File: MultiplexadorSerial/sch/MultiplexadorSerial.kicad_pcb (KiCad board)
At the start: 2 copper layers, 69.2 x 54 mm, 65 parts, among them J1 SL4, J2 SL3, J3 SL1, J4 SL2, Q1 Q_NPN_CBE, Q2 Q_NPN_CBE, Q3 Q_NPN_CBE, Q4 Q_NPN_CBE, U1 SP3481CP, U2 SP3481CP, U3 SP3481CP, U4 SP3481CP, U5 4052

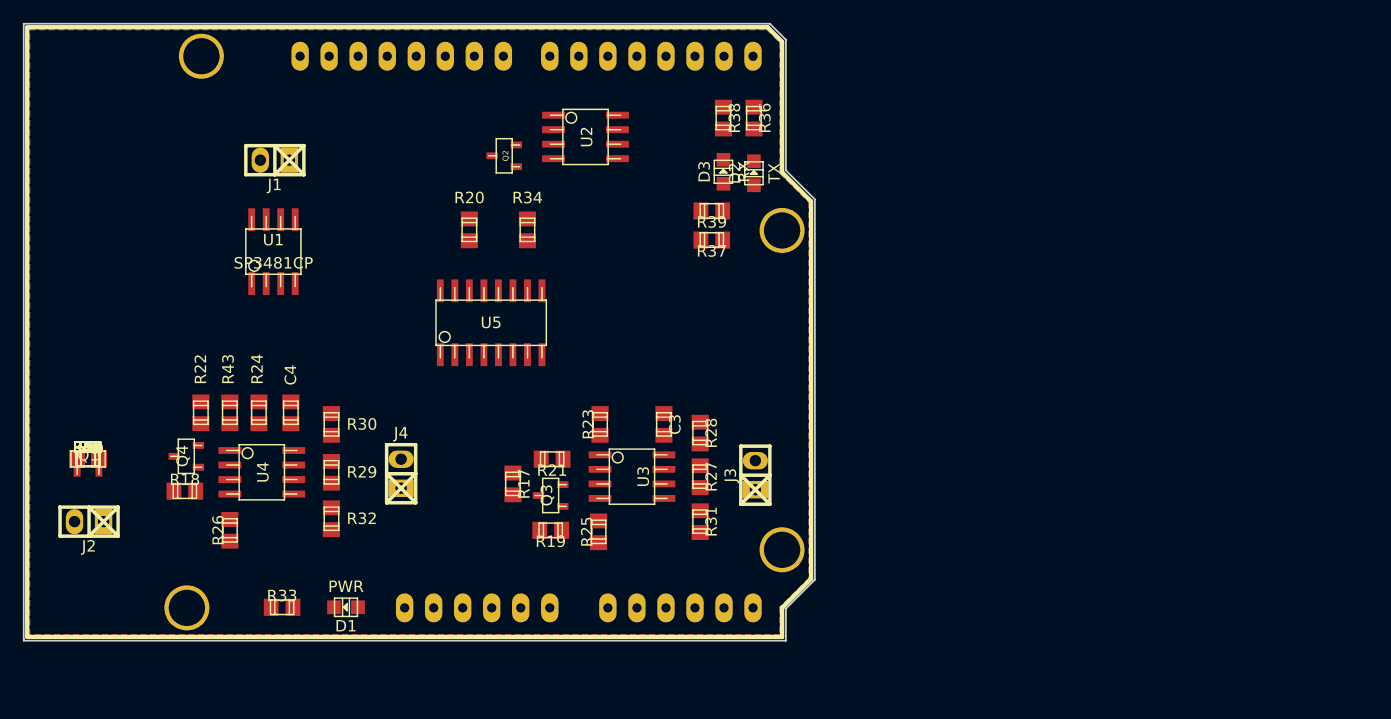
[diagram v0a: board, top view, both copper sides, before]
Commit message: novo desenho
Signed-off-by: cuki2 <mauricio@krebs.com.br>
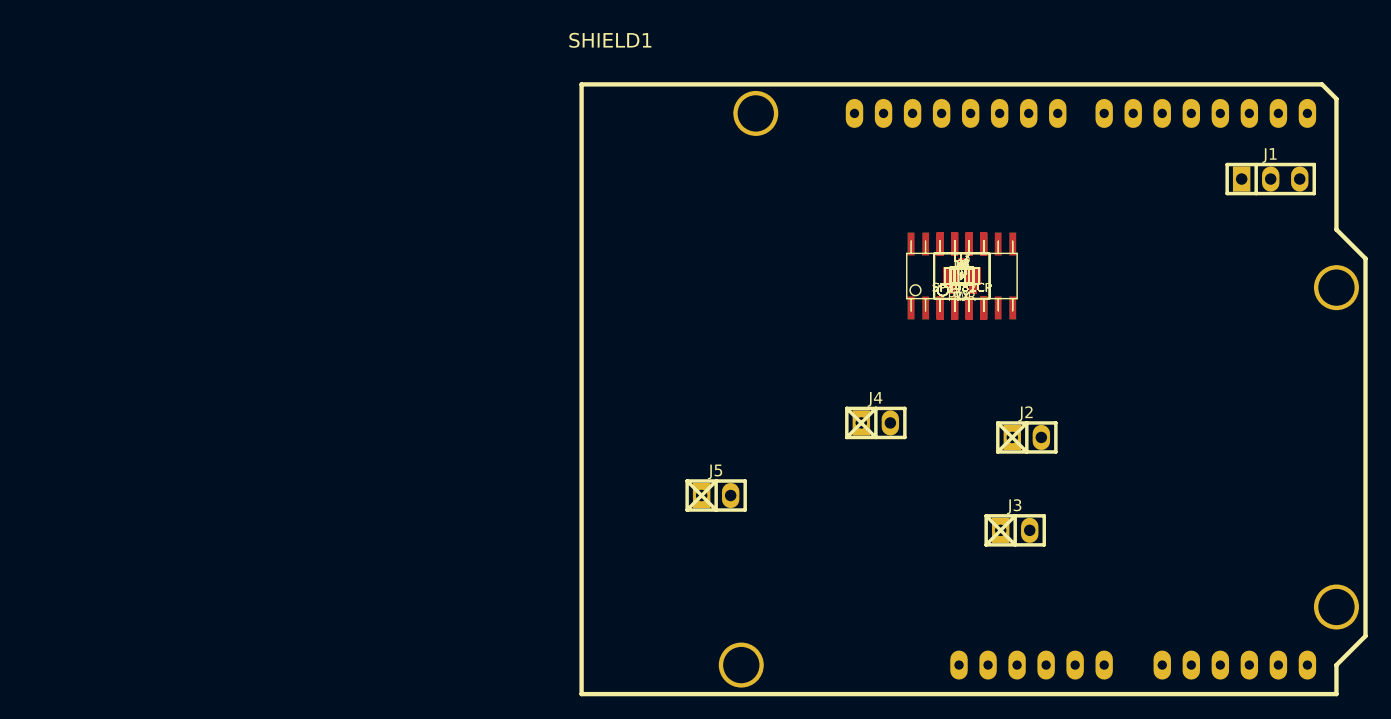
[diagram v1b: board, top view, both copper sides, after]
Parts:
- added J5: SL4, w_pin_strip:pin_socket_2, F.Cu at (160.3, 87.6)
- added R44, R45: 560R, w_smd_resistors:r_0805, F.Cu at (181.8, 68.4)
- D1: value PWR -> TX
- D2: value TX -> PWR
- J1: value SL4 -> SL; footprint w_pin_strip:pin_socket_2 -> w_pin_strip:pin_socket_3
- J2: value SL3 -> SL1
- J3: value SL1 -> SL2
- J4: value SL2 -> SL3
- R1, R2: value 10k -> 1k2
- R10, R18, R26: value 10k -> 560R
- R11, R27: value 120R -> 560R
- R12, R16: value 560R -> 330R
- R13: value 120R -> 330R
- R14, R15, R19, R20, R24, R28, R3, R30, R39, R4, R8: value 560R -> 10k
- R17: value 10k -> 330R
- R22, R40, R41, R6: value 10k -> 360R
- R23, R31, R32, R7: value 560R -> 360R
- R25, R43, R9: value 10k -> 120R
- R29: value 120R -> 10k
- R33, R37: value 1k2 -> 10k
- R34: value 330R -> 120R
- R35, R36: value 330R -> 560R
- R38: value 330R -> 10k
- U2: value SP3481CP -> 4052; footprint w_smd_dil:so-8 -> w_smd_dil:so-16
- U5: value 4052 -> SP3481CP; footprint w_smd_dil:so-16 -> w_smd_dil:so-8
- moved J1 87.1 mm to (208.8, 59.9), turned to 0 degrees
- moved J2 82.4 mm to (187.5, 82.5), turned to 0 degrees
- moved C1 78.1 mm to (181.8, 68.4)
- moved C2 78.1 mm to (181.8, 68.4)
- moved C5 78.1 mm to (181.8, 68.4)
- moved Q1 78.1 mm to (181.8, 68.4)
- moved R1 78.1 mm to (181.8, 68.4)
- moved R10 78.1 mm to (181.8, 68.4)
- moved R11 78.1 mm to (181.8, 68.4)
- moved R12 78.1 mm to (181.8, 68.4)
- moved R13 78.1 mm to (181.8, 68.4)
- moved R14 78.1 mm to (181.8, 68.4)
- moved R15 78.1 mm to (181.8, 68.4)
- moved R16 78.1 mm to (181.8, 68.4)
- moved R2 78.1 mm to (181.8, 68.4)
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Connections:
- C1 pad 1: VDD -> +5V
- C2 pad 1: VDD -> +5V
- C3 pad 1: VDD -> +5V
- C4 pad 1: VDD -> +5V
- C5 pad 1: VDD -> +5V
- D1 pad 1: VDD -> Net-(D1-Pad1)
- D1 pad 2: Net-(D1-Pad2) -> /TX
- D2 pad 1: Net-(D2-Pad1) -> +5V
- J1 pad 1: Net-(J1-Pad1) -> /TX
- J1 pad 2: Net-(J1-Pad2) -> /RX
- R1 pad 1: Net-(Q1-Pad2) -> +5V
- R1 pad 2: Net-(R1-Pad2) -> Net-(D1-Pad1)
- R10 pad 1: Net-(R10-Pad1) -> Net-(J2-Pad2)
- R10 pad 2: VDD -> GND
- R11 pad 1: Net-(J1-Pad1) -> +5V
- R11 pad 2: Net-(J1-Pad2) -> Net-(J2-Pad1)
- R12 pad 1: Net-(J1-Pad2) -> /ADR0
- R12 pad 2: GND -> Net-(R12-Pad2)
- R13 pad 1: Net-(J2-Pad1) -> /ADR1
- R13 pad 2: Net-(J2-Pad2) -> Net-(R13-Pad2)
- R14 pad 1: Net-(J2-Pad2) -> GND
- R14 pad 2: GND -> Net-(R12-Pad2)
- R15 pad 1: VDD -> GND
- R15 pad 2: Net-(J1-Pad1) -> Net-(R13-Pad2)
- R16 pad 1: VDD -> /TX
- R16 pad 2: Net-(J2-Pad1) -> Net-(R16-Pad2)
- R17 pad 1: Net-(Q3-Pad2) -> /RX
- R17 pad 2: Net-(R17-Pad2) -> Net-(D3-Pad2)
- R18 pad 1: Net-(Q4-Pad2) -> +5V
- R18 pad 2: Net-(R18-Pad2) -> Net-(D3-Pad1)
- R19 pad 1: Net-(R17-Pad2) -> Net-(Q2-Pad2)
- R19 pad 2: Net-(R19-Pad2) -> /RX2
- R2 pad 1: Net-(Q2-Pad2) -> GND
- R2 pad 2: Net-(R2-Pad2) -> Net-(D2-Pad2)
- R20 pad 1: Net-(R18-Pad2) -> +5V
- R20 pad 2: Net-(R20-Pad2) -> Net-(Q2-Pad3)
- R21 pad 1: VDD -> /TX2
- R21 pad 2: Net-(Q3-Pad3) -> +5V
- R22 pad 1: VDD -> /RX2
- R22 pad 2: Net-(Q4-Pad3) -> Net-(R22-Pad2)
- R23 pad 1: Net-(R23-Pad1) -> /TX2
- R24 pad 1: Net-(R24-Pad1) -> +5V
- R24 pad 2: Net-(R24-Pad2) -> Net-(R22-Pad2)
- R25 pad 1: Net-(R19-Pad2) -> Net-(J3-Pad1)
- R25 pad 2: VDD -> Net-(J3-Pad2)
- R26 pad 1: Net-(R20-Pad2) -> Net-(J3-Pad2)
- R26 pad 2: VDD -> GND
- R27 pad 1: Net-(J3-Pad1) -> +5V
- R27 pad 2: Net-(J3-Pad2) -> Net-(J3-Pad1)
- R28 pad 1: Net-(J3-Pad2) -> Net-(Q3-Pad2)
- R28 pad 2: GND -> /RX3
- R29 pad 1: Net-(J4-Pad1) -> +5V
- R29 pad 2: Net-(J4-Pad2) -> Net-(Q3-Pad3)
- R3 pad 1: Net-(R1-Pad2) -> Net-(Q1-Pad2)
- R3 pad 2: Net-(R3-Pad2) -> /RX1
- R30 pad 1: Net-(J4-Pad2) -> /TX3
- R30 pad 2: GND -> +5V
- R31 pad 1: VDD -> /RX3
- R31 pad 2: Net-(J3-Pad1) -> Net-(R31-Pad2)
- R32 pad 1: VDD -> /TX3
- R32 pad 2: Net-(J4-Pad1) -> Net-(R32-Pad2)
- R33 pad 1: Net-(D1-Pad2) -> +5V
- R33 pad 2: GND -> Net-(R31-Pad2)
- R34 pad 1: Net-(R34-Pad1) -> Net-(J4-Pad1)
- R34 pad 2: Net-(R34-Pad2) -> Net-(J4-Pad2)
- R35 pad 1: Net-(R35-Pad1) -> Net-(J4-Pad2)
- R35 pad 2: Net-(R35-Pad2) -> GND
- R36 pad 1: Net-(R36-Pad1) -> +5V
- R36 pad 2: Net-(D2-Pad2) -> Net-(J4-Pad1)
- R37 pad 1: VDD -> Net-(Q4-Pad2)
- R37 pad 2: Net-(D2-Pad1) -> /RX4
- R38 pad 1: Net-(D3-Pad2) -> +5V
- R38 pad 2: Net-(R38-Pad2) -> Net-(Q4-Pad3)
- R39 pad 1: VDD -> /TX4
- R39 pad 2: Net-(D3-Pad1) -> +5V
- R4 pad 1: Net-(R2-Pad2) -> +5V
- R4 pad 2: Net-(R10-Pad1) -> Net-(Q1-Pad3)
- R40 pad 1: VDD -> /RX4
- R41 pad 1: VDD -> /TX4
- R42 pad 1: VDD -> +5V
- R42 pad 2: Net-(R23-Pad2) -> Net-(R40-Pad2)
- R43 pad 1: VDD -> Net-(J5-Pad1)
- R43 pad 2: Net-(R24-Pad2) -> Net-(J5-Pad2)
- R5 pad 1: VDD -> /TX1
- R5 pad 2: Net-(Q1-Pad3) -> +5V
- R6 pad 1: VDD -> /RX1
- R6 pad 2: Net-(Q2-Pad3) -> Net-(R6-Pad2)
- R7 pad 1: Net-(R7-Pad1) -> /TX1
- R7 pad 2: Net-(R40-Pad2) -> Net-(R7-Pad2)
- R8 pad 1: Net-(R8-Pad1) -> +5V
- R8 pad 2: Net-(R41-Pad2) -> Net-(R6-Pad2)
- R9 pad 1: Net-(R3-Pad2) -> Net-(J2-Pad1)
- R9 pad 2: VDD -> Net-(J2-Pad2)
- SHIELD1 pad 0: Net-(D2-Pad2) -> /RX
- SHIELD1 pad 1: Net-(R38-Pad2) -> /TX
- SHIELD1 pad 5V: VDD -> +5V
- SHIELD1 pad AD0: Net-(R34-Pad2) -> /ADR0
- SHIELD1 pad AD1: Net-(R35-Pad2) -> /ADR1
- U1 pad 1: Net-(R40-Pad2) -> Net-(R6-Pad2)
- U1 pad 4: Net-(R3-Pad2) -> Net-(R7-Pad2)
- U1 pad 6: Net-(J1-Pad1) -> Net-(J2-Pad1)
- U1 pad 7: Net-(J1-Pad2) -> Net-(J2-Pad2)
- U1 pad 8: VDD -> +5V
- U2 pad 1: Net-(R41-Pad2) -> /RX1
- U2 pad 2: Net-(Q2-Pad3) -> /RX3
- U2 pad 3: Net-(Q2-Pad3) -> Net-(D3-Pad2)
- U2 pad 4: Net-(R10-Pad1) -> /RX4
- U2 pad 5: GND -> /RX2
- U2 pad 6: Net-(J2-Pad1) -> GND
- U2 pad 7: Net-(J2-Pad2) -> GND
- U2 pad 8: VDD -> GND
- U3 pad 1: Net-(R23-Pad2) -> Net-(R22-Pad2)
- U3 pad 2: Net-(Q3-Pad3) -> Net-(Q2-Pad3)
- U3 pad 3: Net-(Q3-Pad3) -> Net-(Q2-Pad3)
- U3 pad 4: Net-(R19-Pad2) -> Net-(R23-Pad2)
- U3 pad 8: VDD -> +5V
- U4 pad 1: Net-(R24-Pad2) -> Net-(R31-Pad2)
- U4 pad 2: Net-(Q4-Pad3) -> Net-(Q3-Pad3)
- U4 pad 3: Net-(Q4-Pad3) -> Net-(Q3-Pad3)
- U4 pad 4: Net-(R20-Pad2) -> Net-(R32-Pad2)
- U4 pad 8: VDD -> +5V
- U5 pad 1: Net-(R23-Pad1) -> Net-(R40-Pad2)
- U5 pad 2: Net-(R7-Pad1) -> Net-(Q4-Pad3)
- U5 pad 3: Net-(R36-Pad1) -> Net-(Q4-Pad3)
- U5 pad 4: Net-(R8-Pad1) -> Net-(R41-Pad2)
- U5 pad 5: Net-(R24-Pad1) -> GND
- U5 pad 6: GND -> Net-(J5-Pad1)
- U5 pad 7: GND -> Net-(J5-Pad2)
- U5 pad 8: GND -> +5V
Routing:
- removed copper zone on B.Cu, net GND
- removed copper zone on F.Cu, net GND
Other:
- board outline removed
